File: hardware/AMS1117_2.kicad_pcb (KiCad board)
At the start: 2 copper layers, 9 parts, among them J13 Conn_01x03, U5 AMS1117-3.3

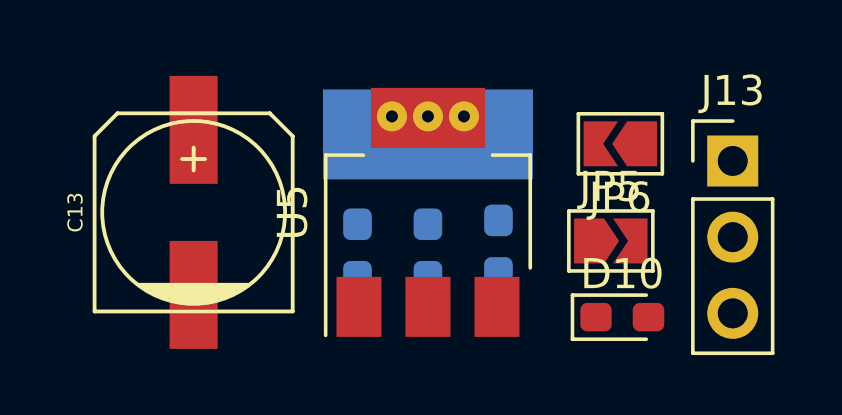
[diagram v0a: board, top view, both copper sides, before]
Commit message: update,
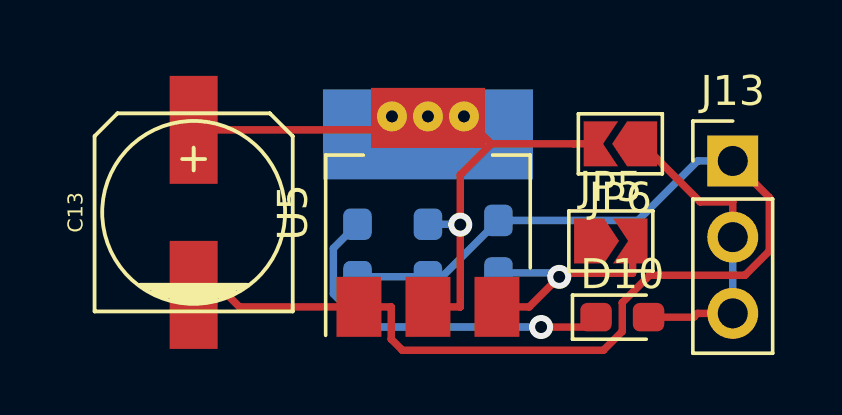
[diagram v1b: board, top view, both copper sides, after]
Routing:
- net GND: track 0.00 -> 40.1 mm
- net Net-(C12-Pad1): track 0.00 -> 22.1 mm, vias 0 -> 1
- net Net-(D10-Pad1): track 0.00 -> 12.0 mm, vias 0 -> 1
- net Vb: track 0.00 -> 10.4 mm
- net Net-(C11-Pad1): track 0.00 -> 8.14 mm, vias 0 -> 1
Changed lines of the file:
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@@
     (thickness 1.6)
     (drawings 0)
-    (tracks 0)
+    (tracks 60)
     (zones 0)
     (modules 9)
@@
     (uvia_dia 0.3)
     (uvia_drill 0.1)
-    (add_net +5V)
     (add_net GND)
     (add_net "Net-(C11-Pad1)")
@@
     )
   )
+  (segment (start 24.13 21.223) (end 22.253 23.1) (width 0.25) (layer B.Cu) (net 1))
+  (segment (start 22.253 23.1) (end 21.7805 23.1) (width 0.25) (layer B.Cu) (net 1))
+  (segment (start 30.7652 19.2405) (end 28.7827 21.223) (width 0.25) (layer B.Cu) (net 1))
+  (segment (start 28.7827 21.223) (end 24.13 21.223) (width 0.25) (layer B.Cu) (net 1))
+  (segment (start 19.4805 24.105) (end 20.5558 24.105) (width 0.25) (layer F.Cu) (net 1))
+  (segment (start 20.5558 24.105) (end 20.5558 25.1803) (width 0.25) (layer F.Cu) (net 1))
+  (segment (start 20.5558 25.1803) (end 20.9258 25.5503) (width 0.25) (layer F.Cu) (net 1))
+  (segment (start 20.9258 25.5503) (end 27.6294 25.5503) (width 0.25) (layer F.Cu) (net 1))
+  (segment (start 27.6294 25.5503) (end 28.2575 24.9222) (width 0.25) (layer F.Cu) (net 1))
+  (segment (start 28.2575 24.9222) (end 28.2575 23.9637) (width 0.25) (layer F.Cu) (net 1))
+  (segment (start 28.2575 23.9637) (end 29.1707 23.0505) (width 0.25) (layer F.Cu) (net 1))
+  (segment (start 29.1707 23.0505) (end 32.3507 23.0505) (width 0.25) (layer F.Cu) (net 1))
+  (segment (start 32.3507 23.0505) (end 33.158 22.2432) (width 0.25) (layer F.Cu) (net 1))
+  (segment (start 33.158 22.2432) (end 33.158 20.458) (width 0.25) (layer F.Cu) (net 1))
+  (segment (start 33.158 20.458) (end 31.9405 19.2405) (width 0.25) (layer F.Cu) (net 1))
+  (segment (start 15.0954 23.7058) (end 15.4946 24.105) (width 0.25) (layer F.Cu) (net 1))
+  (segment (start 15.4946 24.105) (end 19.4805 24.105) (width 0.25) (layer F.Cu) (net 1))
+  (segment (start 21.7805 23.1) (end 19.431 23.1) (width 0.25) (layer B.Cu) (net 1))
+  (segment (start 31.9405 19.2405) (end 30.7652 19.2405) (width 0.25) (layer B.Cu) (net 1))
+  (segment (start 13.97 23.7058) (end 15.0954 23.7058) (width 0.25) (layer F.Cu) (net 1))
+  (segment (start 28.6015 22.9828) (end 26.278 22.9828) (width 0.25) (layer F.Cu) (net 2))
+  (segment (start 26.278 22.9828) (end 26.1565 23.1043) (width 0.25) (layer F.Cu) (net 2))
+  (segment (start 25.1558 24.105) (end 26.1564 23.1044) (width 0.25) (layer F.Cu) (net 2))
+  (segment (start 26.1564 23.1044) (end 26.1564 23.1043) (width 0.25) (layer F.Cu) (net 2))
+  (segment (start 26.1564 23.1043) (end 26.1565 23.1043) (width 0.25) (layer F.Cu) (net 2))
+  (segment (start 24.13 22.973) (end 26.0252 22.973) (width 0.25) (layer B.Cu) (net 2))
+  (segment (start 26.0252 22.973) (end 26.1565 23.1043) (width 0.25) (layer B.Cu) (net 2))
+  (segment (start 24.0805 24.105) (end 25.1558 24.105) (width 0.25) (layer F.Cu) (net 2))
+  (segment (start 28.6015 21.9075) (end 28.6015 22.9828) (width 0.25) (layer F.Cu) (net 2))
+  (via (at 26.1565 23.1043) (size 0.8) (layers F.Cu B.Cu) (net 2))
+  (segment (start 23.8945 18.669) (end 22.9805 17.755) (width 0.25) (layer F.Cu) (net 3))
+  (segment (start 26.6437 18.669) (end 23.8945 18.669) (width 0.25) (layer F.Cu) (net 3))
+  (segment (start 22.8579 21.3635) (end 22.8579 19.7056) (width 0.25) (layer F.Cu) (net 3))
+  (segment (start 22.8579 19.7056) (end 23.8945 18.669) (width 0.25) (layer F.Cu) (net 3))
+  (segment (start 22.8558 24.105) (end 22.8579 24.1029) (width 0.25) (layer F.Cu) (net 3))
+  (segment (start 22.8579 24.1029) (end 22.8579 21.3635) (width 0.25) (layer F.Cu) (net 3))
+  (segment (start 21.7805 21.35) (end 22.8444 21.35) (width 0.25) (layer B.Cu) (net 3))
+  (segment (start 22.8444 21.35) (end 22.8579 21.3635) (width 0.25) (layer B.Cu) (net 3))
+  (segment (start 21.7805 24.105) (end 22.8558 24.105) (width 0.25) (layer F.Cu) (net 3))
+  (segment (start 21.7805 17.755) (end 22.9805 17.755) (width 0.25) (layer F.Cu) (net 3))
+  (segment (start 20.5805 17.755) (end 21.7805 17.755) (width 0.25) (layer F.Cu) (net 3))
+  (segment (start 27.469 18.669) (end 26.6437 18.669) (width 0.25) (layer F.Cu) (net 3))
+  (segment (start 21.7805 17.805) (end 21.7805 17.755) (width 0.25) (layer F.Cu) (net 3))
+  (segment (start 13.97 18.2042) (end 20.1313 18.2042) (width 0.25) (layer F.Cu) (net 3))
+  (segment (start 20.1313 18.2042) (end 20.5805 17.755) (width 0.25) (layer F.Cu) (net 3))
+  (via (at 22.8579 21.3635) (size 0.8) (layers F.Cu B.Cu) (net 3))
+  (segment (start 31.9405 21.7805) (end 31.9405 20.6052) (width 0.25) (layer F.Cu) (net 4))
+  (segment (start 31.9405 20.6052) (end 30.8552 20.6052) (width 0.25) (layer F.Cu) (net 4))
+  (segment (start 30.8552 20.6052) (end 28.919 18.669) (width 0.25) (layer F.Cu) (net 4))
+  (segment (start 31.9405 21.7805) (end 31.9405 24.3205) (width 0.25) (layer B.Cu) (net 4))
+  (segment (start 31.9405 24.3205) (end 30.7652 24.3205) (width 0.25) (layer F.Cu) (net 4))
+  (segment (start 29.1325 24.4475) (end 30.6382 24.4475) (width 0.25) (layer F.Cu) (net 4))
+  (segment (start 30.6382 24.4475) (end 30.7652 24.3205) (width 0.25) (layer F.Cu) (net 4))
+  (segment (start 27.3825 24.4475) (end 27.0535 24.7765) (width 0.25) (layer F.Cu) (net 5))
+  (segment (start 27.0535 24.7765) (end 25.5522 24.7765) (width 0.25) (layer F.Cu) (net 5))
+  (segment (start 19.431 21.35) (end 18.6276 22.1534) (width 0.25) (layer B.Cu) (net 5))
+  (segment (start 18.6276 22.1534) (end 18.6276 23.6707) (width 0.25) (layer B.Cu) (net 5))
+  (segment (start 18.6276 23.6707) (end 19.7334 24.7765) (width 0.25) (layer B.Cu) (net 5))
+  (segment (start 19.7334 24.7765) (end 25.5522 24.7765) (width 0.25) (layer B.Cu) (net 5))
+  (via (at 25.5522 24.7765) (size 0.8) (layers F.Cu B.Cu) (net 5))
 )
